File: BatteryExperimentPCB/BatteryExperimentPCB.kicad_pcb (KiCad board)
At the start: 2 copper layers, 27.8 x 32.5 mm, 32 parts, among them J1 TYPE-C-31-M-12, J2 Conn_01x12_Pin, J3 Conn_01x12_Pin, Q1 DMG1012T, SW1 K2-1157SP, U1 ATtiny3226-M, U2 USBLC6-2P6, U3 BQ25628RYKR

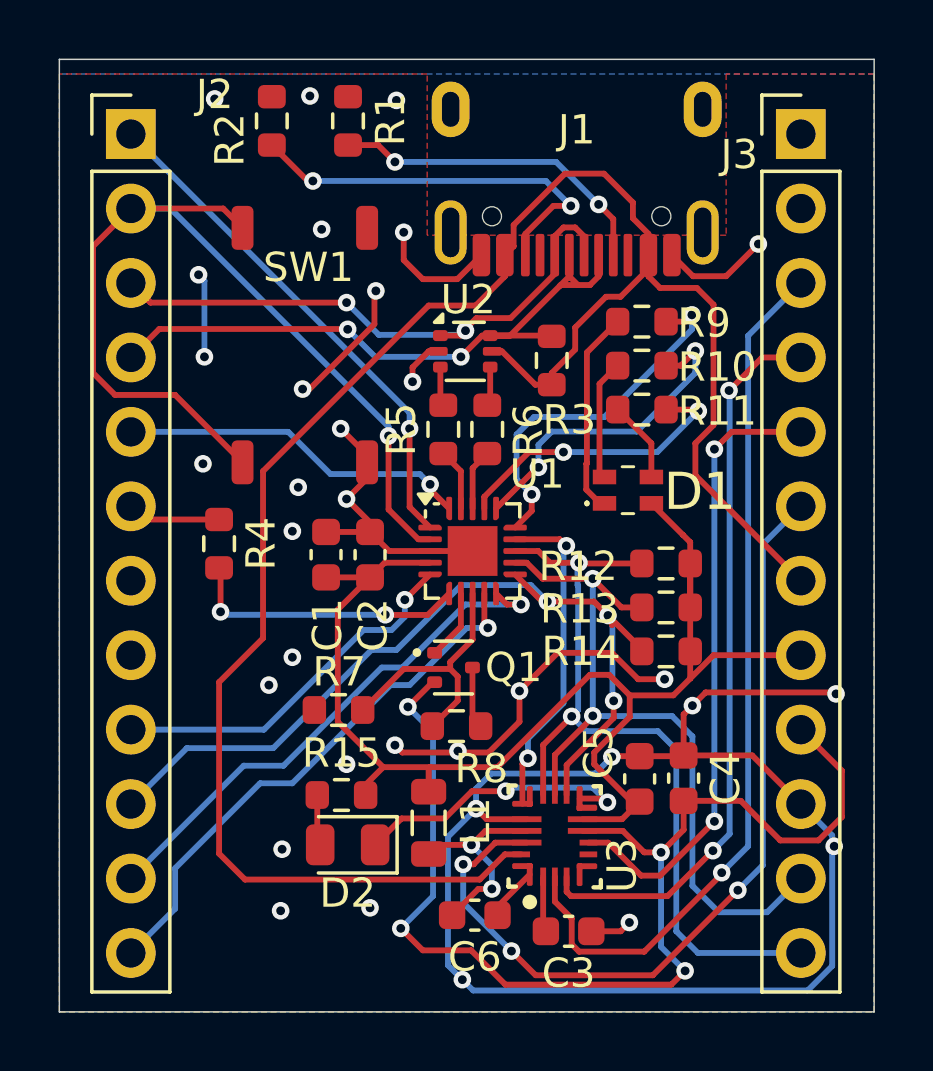
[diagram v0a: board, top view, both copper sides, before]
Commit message: cleanup
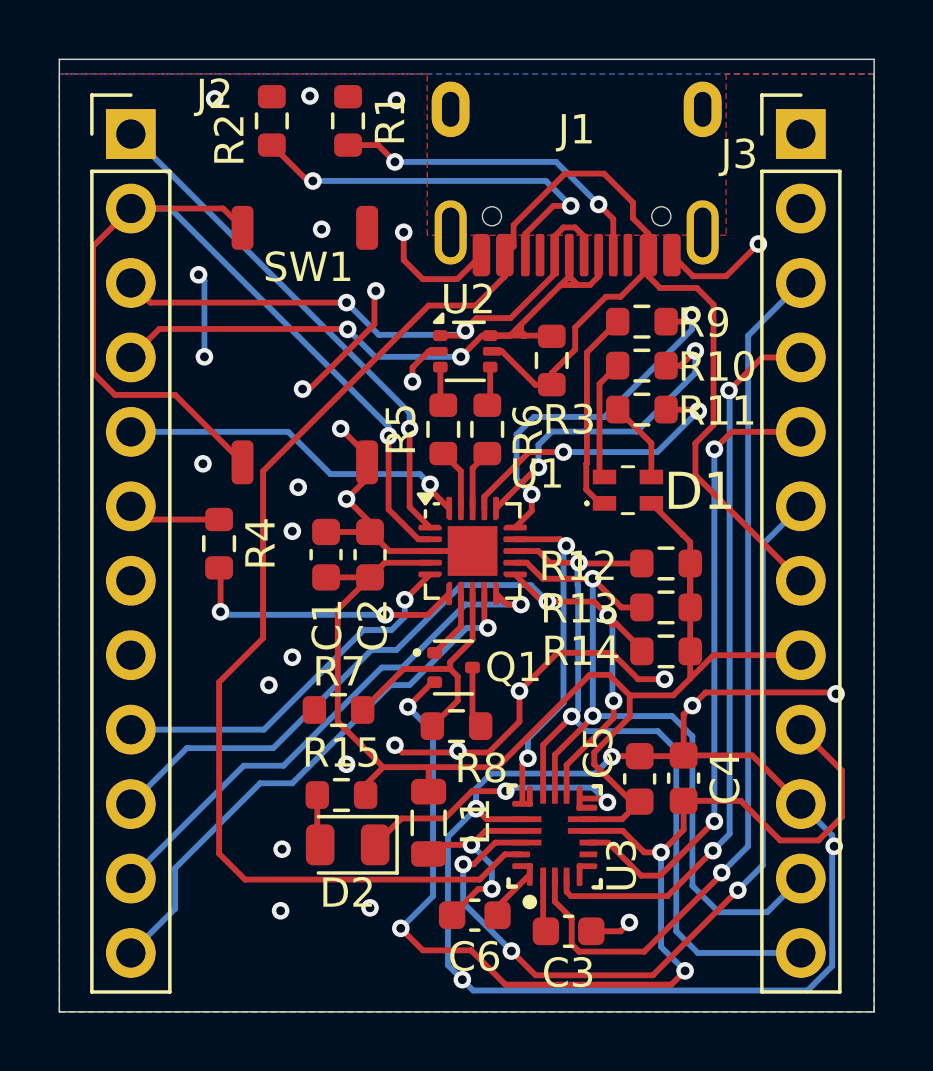
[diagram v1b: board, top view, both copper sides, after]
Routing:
- net DBUS-: track 22.3 -> 23.4 mm
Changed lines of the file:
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@@
+	)
+	(segment
+		(start 225 63.875)
+		(end 225 63.85)
+		(width 0.2)
+		(layer "F.Cu")
+		(net 12)
+	)
+	(segment
+		(start 224.9525 63.8025)
+		(end 224.9525 63.5025)
+		(width 0.2)
+		(layer "F.Cu")
+		(net 12)
 	)
 	(segment
 		(start 219.037696 63.662304)
 		(end 219.025392 63.65)
+		(width 0.2)
+		(layer "F.Cu")
+		(net 12)
+	)
+	(segment
+		(start 225 63.875)
+		(end 225.1 63.875)
+		(width 0.2)
+		(layer "F.Cu")
+		(net 12)
+	)
+	(segment
+		(start 223.9 63.875)
+		(end 225 63.875)
 		(width 0.2)
 		(layer "F.Cu")
@@
 	)
 	(segment
+		(start 224.8525 63.6275)
+		(end 225.1 63.875)
+		(width 0.2)
+		(layer "F.Cu")
+		(net 12)
+	)
+	(segment
 		(start 226.895001 62.15)
 		(end 226.305 62.15)
+		(width 0.2)
+		(layer "F.Cu")
+		(net 12)
+	)
+	(segment
+		(start 224.579999 63.875)
+		(end 224.8025 63.6525)
 		(width 0.2)
 		(layer "F.Cu")
@@
 	)
 	(segment
-		(start 224.579999 63.875)
-		(end 226.2775 62.1775)
-		(width 0.2)
-		(layer "F.Cu")
-		(net 12)
-	)
-	(segment
 		(start 227.6 61.13)
 		(end 227.6 61.854999)
@@
 		(start 226.895001 62.15)
 		(end 226.6 61.854999)
+		(width 0.2)
+		(layer "F.Cu")
+		(net 12)
+	)
+	(segment
+		(start 225.1 63.875)
+		(end 225.975 63.875)
+		(width 0.2)
+		(layer "F.Cu")
+		(net 12)
+	)
+	(segment
+		(start 224.8525 63.6025)
+		(end 224.8525 63.6275)
 		(width 0.2)
 		(layer "F.Cu")
@@
 	)
 	(segment
+		(start 224.8025 63.6525)
+		(end 224.8525 63.6025)
+		(width 0.2)
+		(layer "F.Cu")
+		(net 12)
+	)
+	(segment
 		(start 226.6 61.854999)
 		(end 226.6 61.13)
+		(width 0.2)
+		(layer "F.Cu")
+		(net 12)
+	)
+	(segment
+		(start 225 63.85)
+		(end 224.8025 63.6525)
 		(width 0.2)
 		(layer "F.Cu")
@@
 	)
 	(segment
-		(start 223.9 63.875)
-		(end 225.975 63.875)
+		(start 224.9525 63.5025)
+		(end 226.2775 62.1775)
 		(width 0.2)
 		(layer "F.Cu")
+		(net 12)
+	)
+	(segment
+		(start 224.8525 63.6025)
+		(end 224.9525 63.5025)
+		(width 0.2)
+		(layer "F.Cu")
+		(net 12)
+	)
+	(segment
+		(start 225 63.85)
+		(end 224.9525 63.8025)
+		(width 0.2)
+		(layer "F.Cu")
